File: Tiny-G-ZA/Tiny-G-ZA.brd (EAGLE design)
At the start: 67.9 x 80.6 mm, 44 parts, among them IC1 FT230XS, IC2 LD117ADT-TR, SW1 SPST_TACT-EVQQ2, U1 ATXMEGA192A3-AU

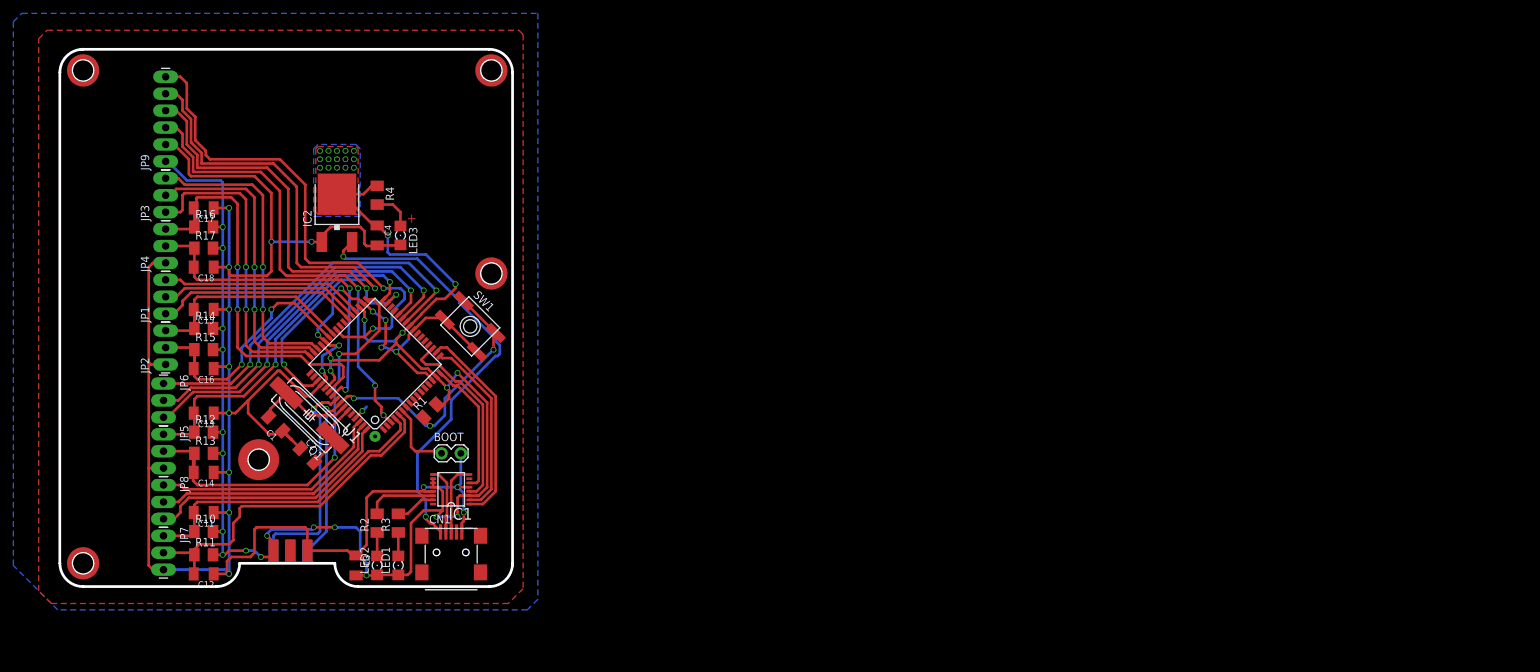
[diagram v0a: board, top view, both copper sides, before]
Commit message: Halfway through RAMPS 1.5 wishlist
Halfway through RAMPS 1.5 wishlist
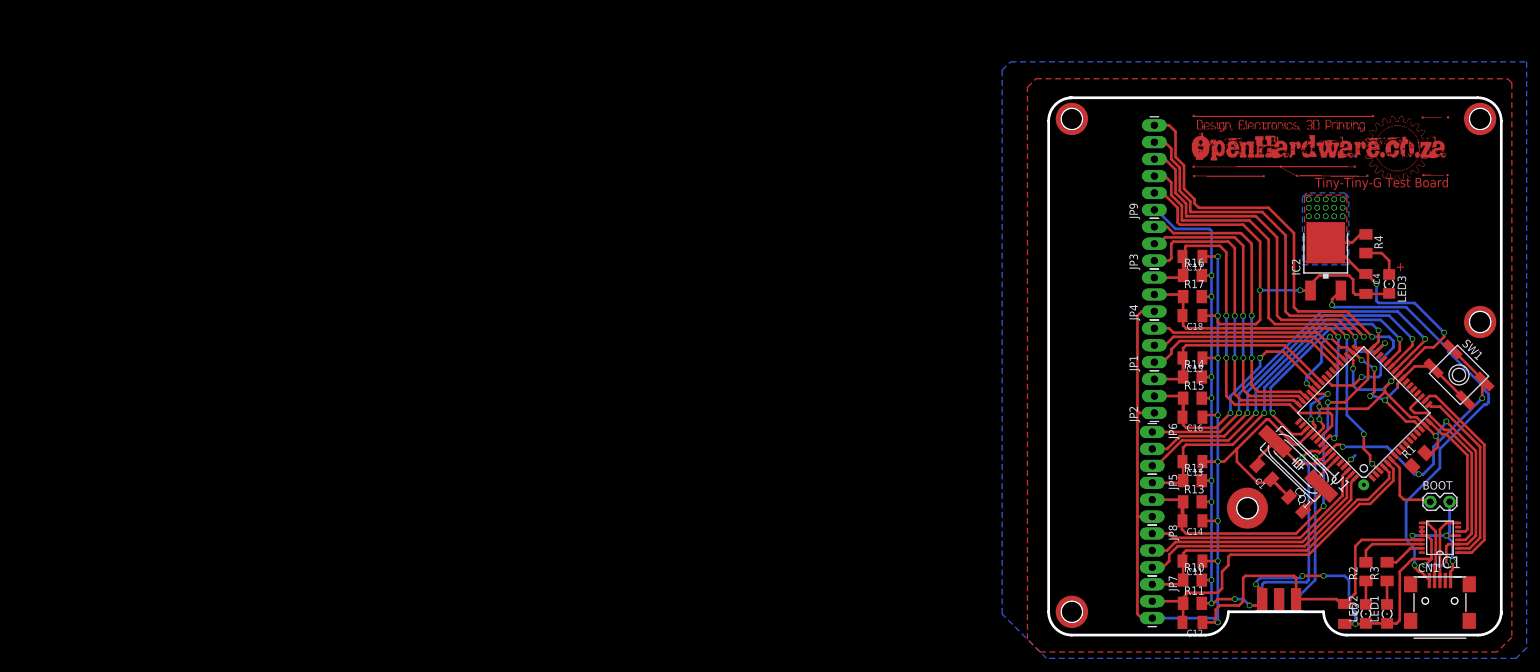
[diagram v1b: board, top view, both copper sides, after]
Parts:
- moved BOOT 148.6 mm to (201.1, 12.7)
- moved C11 148.6 mm to (165.2, 3.83)
- moved C12 148.6 mm to (165.2, -5.38)
- moved C13 148.6 mm to (165.2, 18.8)
- moved C14 148.6 mm to (165.2, 9.86)
- moved C15 148.6 mm to (165.2, 34.3)
- moved C16 148.6 mm to (165.2, 25.4)
- moved C17 148.6 mm to (165.2, 49.6)
- moved C18 148.6 mm to (165.2, 40.7)
- moved C2 148.6 mm to (180.8, 12.4)
- moved C4 148.6 mm to (191.3, 45.4)
- moved CN1 148.6 mm to (202.4, -3.15)
- moved IC1 148.6 mm to (202.4, 7.32)
- moved IC2 148.6 mm to (185.2, 49.2)
- moved JP5 148.6 mm to (159.2, 15.6)
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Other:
- board text added: "0.22u"
- board text added: "150R"
- board text added: "2K7"
- board text added: "56K"
- board text added: "PWR"
- board text added: "Tiny-Tiny-G Test Board"
